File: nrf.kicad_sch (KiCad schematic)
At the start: 25 parts, among them J1 USB_C_Receptacle_USB2.0_16P, SW1 RESET, U1 nRF52840, U2 BQ25101YFPR, Y1 32.768kHz, Y2 32mHz

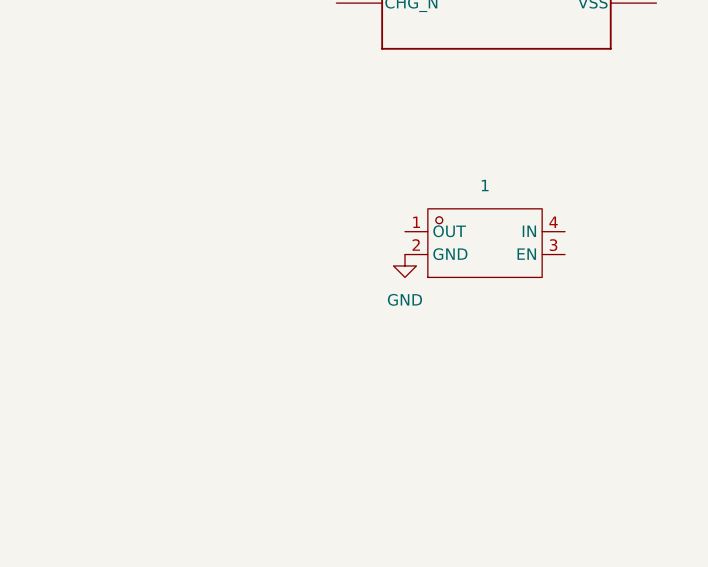
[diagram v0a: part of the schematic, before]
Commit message: Test integracji windows linux
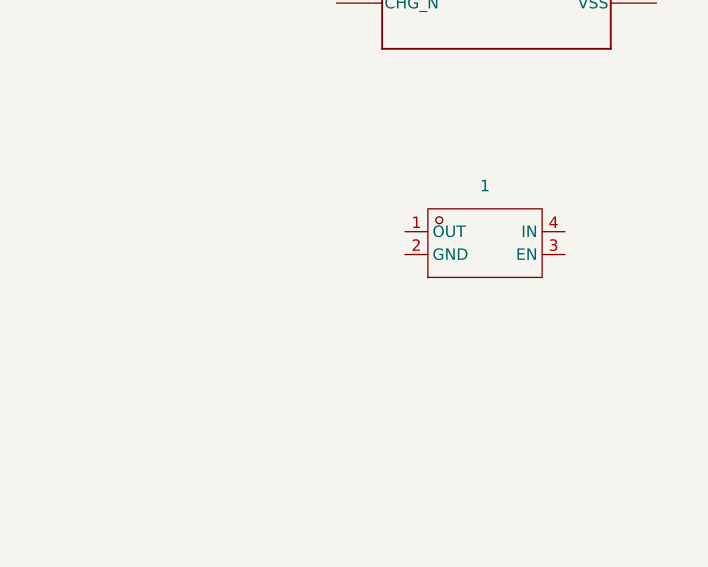
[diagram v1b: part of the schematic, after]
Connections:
- net GND: no longer 1.2 (GND)
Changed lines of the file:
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@@
-	)
-	(symbol
-		(lib_id "power:GND")
-		(at 208.28 87.63 0)
-		(unit 1)
-		(body_style 1)
-		(exclude_from_sim no)
-		(in_bom yes)
-		(on_board yes)
-		(in_pos_files yes)
-		(dnp no)
-		(fields_autoplaced yes)
-		(property "Reference" "#PWR021"
-			(at 208.28 93.98 0)
-			(hide yes)
-			(show_name no)
-			(do_not_autoplace no)
-			(effects
-				(font
-					(size 1.27 1.27)
-				)
-			)
-		)
-		(property "Value" "GND"
-			(at 208.28 92.71 0)
-			(show_name no)
-			(do_not_autoplace no)
-			(effects
-				(font
-					(size 1.27 1.27)
-				)
-			)
-		)
-		(property "Footprint" ""
-			(at 208.28 87.63 0)
-			(hide yes)
-			(show_name no)
-			(do_not_autoplace no)
-			(effects
-				(font
-					(size 1.27 1.27)
-				)
-			)
-		)
-		(property "Datasheet" ""
-			(at 208.28 87.63 0)
-			(hide yes)
-			(show_name no)
-			(do_not_autoplace no)
-			(effects
-				(font
-					(size 1.27 1.27)
-				)
-			)
-		)
-		(property "Description" "Power symbol creates a global label with name \"GND\" , ground"
-			(at 208.28 87.63 0)
-			(hide yes)
-			(show_name no)
-			(do_not_autoplace no)
-			(effects
-				(font
-					(size 1.27 1.27)
-				)
-			)
-		)
-		(pin "1"
-		)
-		(instances
-			(project "nrf"
-				(path "/0c64da4f-9d5f-4fc8-ac76-7e5704c1497b"
-					(reference "#PWR021")
-					(unit 1)
-				)
-			)
-		)
 	)
 	(symbol

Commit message: Test na windows
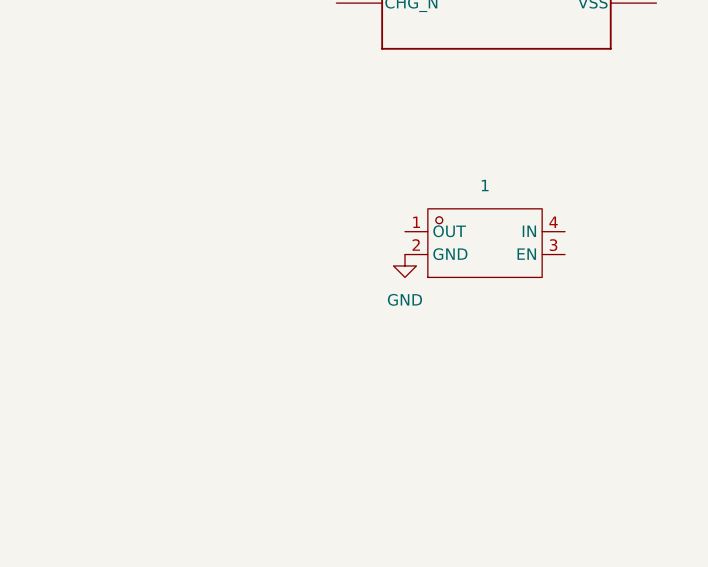
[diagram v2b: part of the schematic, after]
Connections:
- net GND: now also 1.2 (GND)
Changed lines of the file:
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@@
+	)
+	(symbol
+		(lib_id "power:GND")
+		(at 208.28 87.63 0)
+		(unit 1)
+		(body_style 1)
+		(exclude_from_sim no)
+		(in_bom yes)
+		(on_board yes)
+		(in_pos_files yes)
+		(dnp no)
+		(fields_autoplaced yes)
+		(property "Reference" "#PWR021"
+			(at 208.28 93.98 0)
+			(hide yes)
+			(show_name no)
+			(do_not_autoplace no)
+			(effects
+				(font
+					(size 1.27 1.27)
+				)
+			)
+		)
+		(property "Value" "GND"
+			(at 208.28 92.71 0)
+			(show_name no)
+			(do_not_autoplace no)
+			(effects
+				(font
+					(size 1.27 1.27)
+				)
+			)
+		)
+		(property "Footprint" ""
+			(at 208.28 87.63 0)
+			(hide yes)
+			(show_name no)
+			(do_not_autoplace no)
+			(effects
+				(font
+					(size 1.27 1.27)
+				)
+			)
+		)
+		(property "Datasheet" ""
+			(at 208.28 87.63 0)
+			(hide yes)
+			(show_name no)
+			(do_not_autoplace no)
+			(effects
+				(font
+					(size 1.27 1.27)
+				)
+			)
+		)
+		(property "Description" "Power symbol creates a global label with name \"GND\" , ground"
+			(at 208.28 87.63 0)
+			(hide yes)
+			(show_name no)
+			(do_not_autoplace no)
+			(effects
+				(font
+					(size 1.27 1.27)
+				)
+			)
+		)
+		(pin "1"
+		)
+		(instances
+			(project "nrf"
+				(path "/0c64da4f-9d5f-4fc8-ac76-7e5704c1497b"
+					(reference "#PWR021")
+					(unit 1)
+				)
+			)
+		)
 	)
 	(symbol
